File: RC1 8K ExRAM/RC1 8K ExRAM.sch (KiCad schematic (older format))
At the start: 32 parts, among them J1 Expansion, J2 ADDRESS, U1 74LS138, U2 74LS00, U3 74HC595, U4 74HC595, U5 HM62256BLP-7, U6 74LS244, U7 74LS244, U8 74LS245

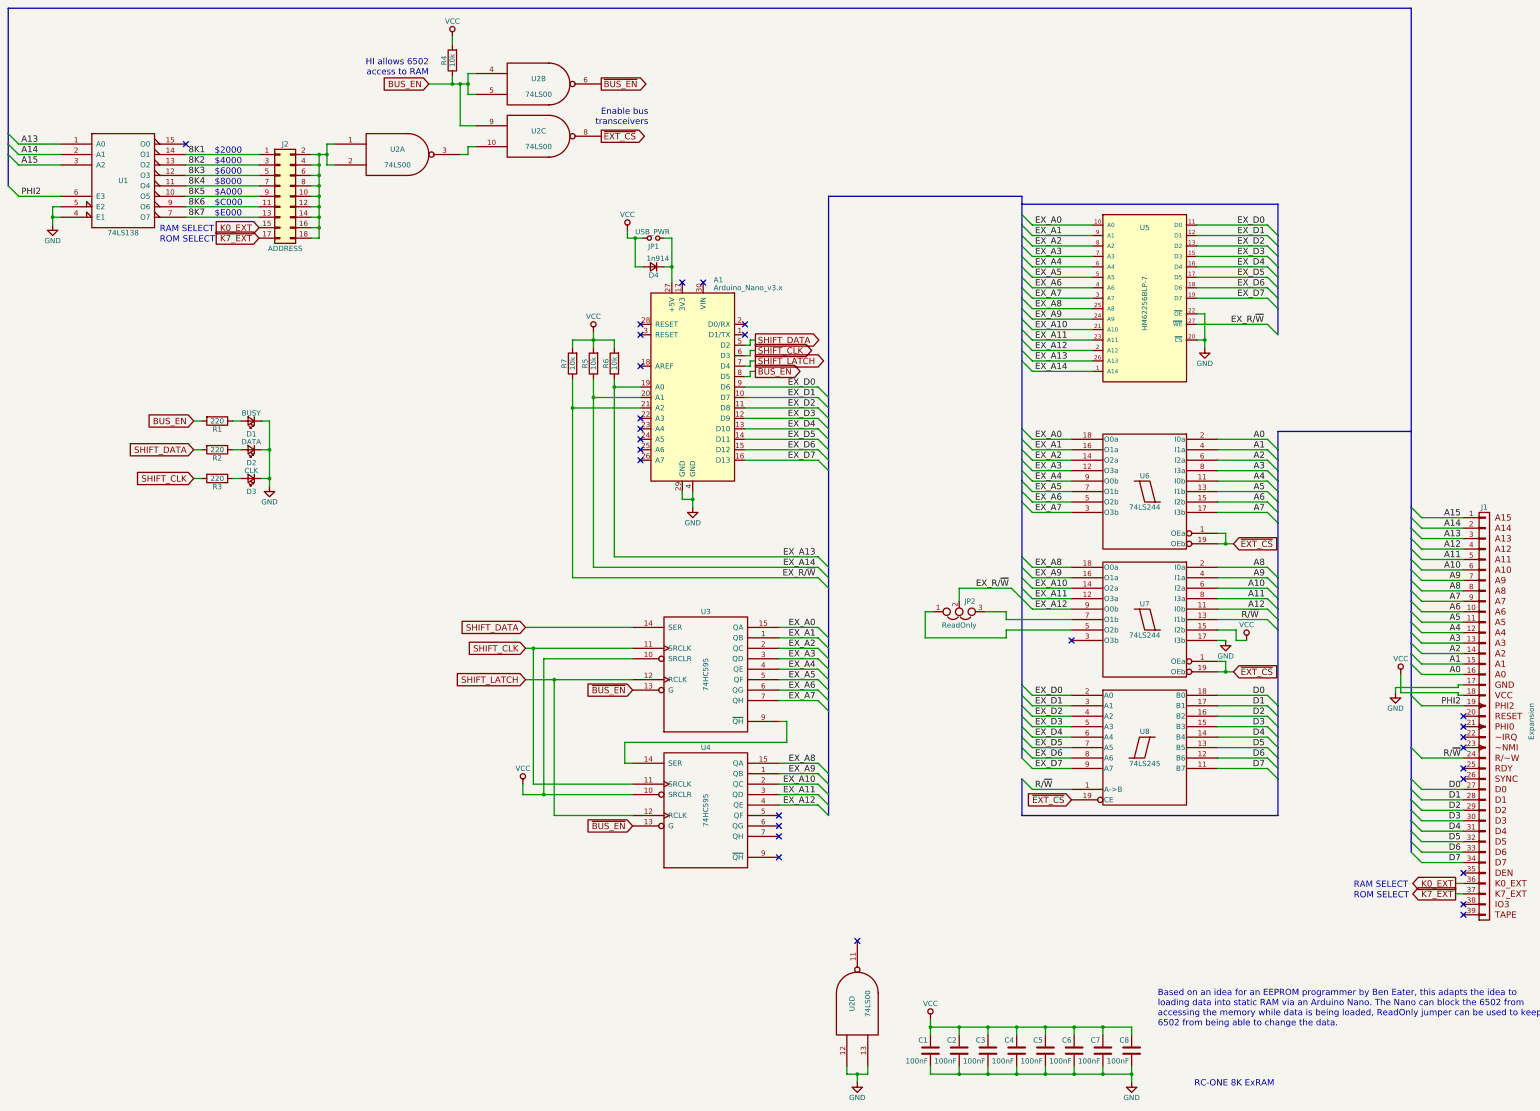
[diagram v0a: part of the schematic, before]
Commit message: Gerber export
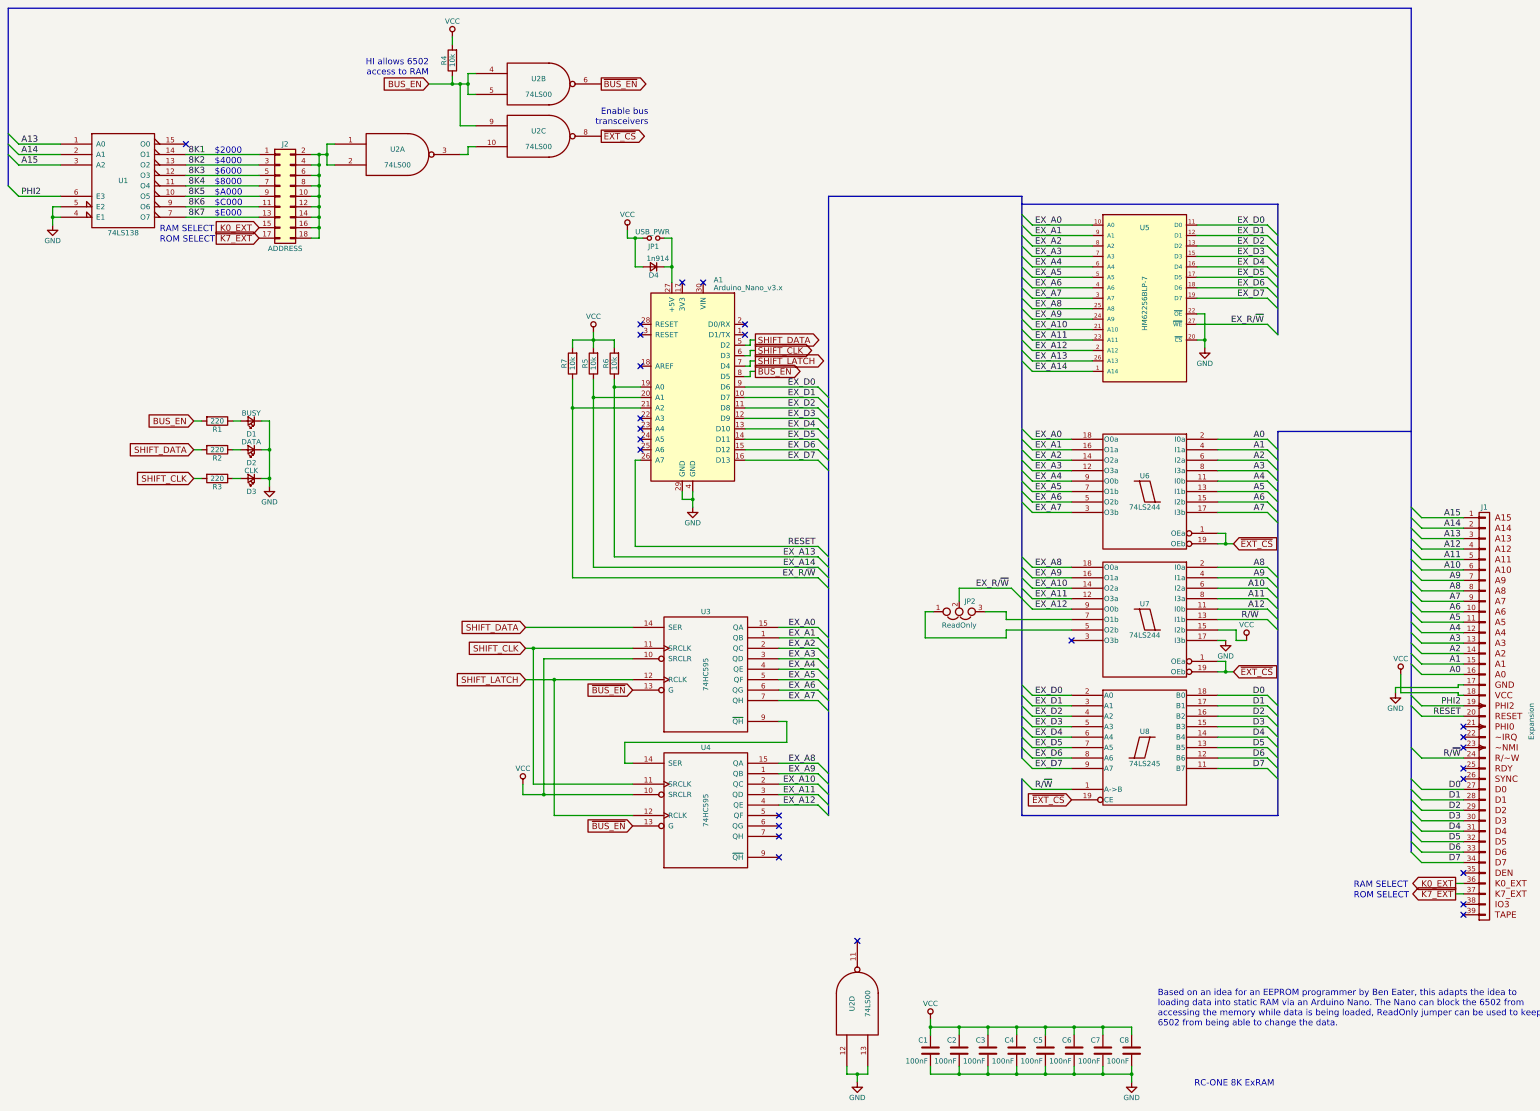
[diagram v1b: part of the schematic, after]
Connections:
- net RESET: now reaches J1.20 (RESET)
- net RESET: now also A1.26 (A7)
- no-connect marks 28 -> 26
